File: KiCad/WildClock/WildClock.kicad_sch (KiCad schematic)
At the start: 33 parts, among them Q1 CA1, Q2 CA2, Q3 CA3, Q4 CA4, SW1 SWUP, SW2 SWDOWN, SW3 SWOK, U1 ESP32-C3-MINI-1, U3 74HC595, U4 TiltSensor

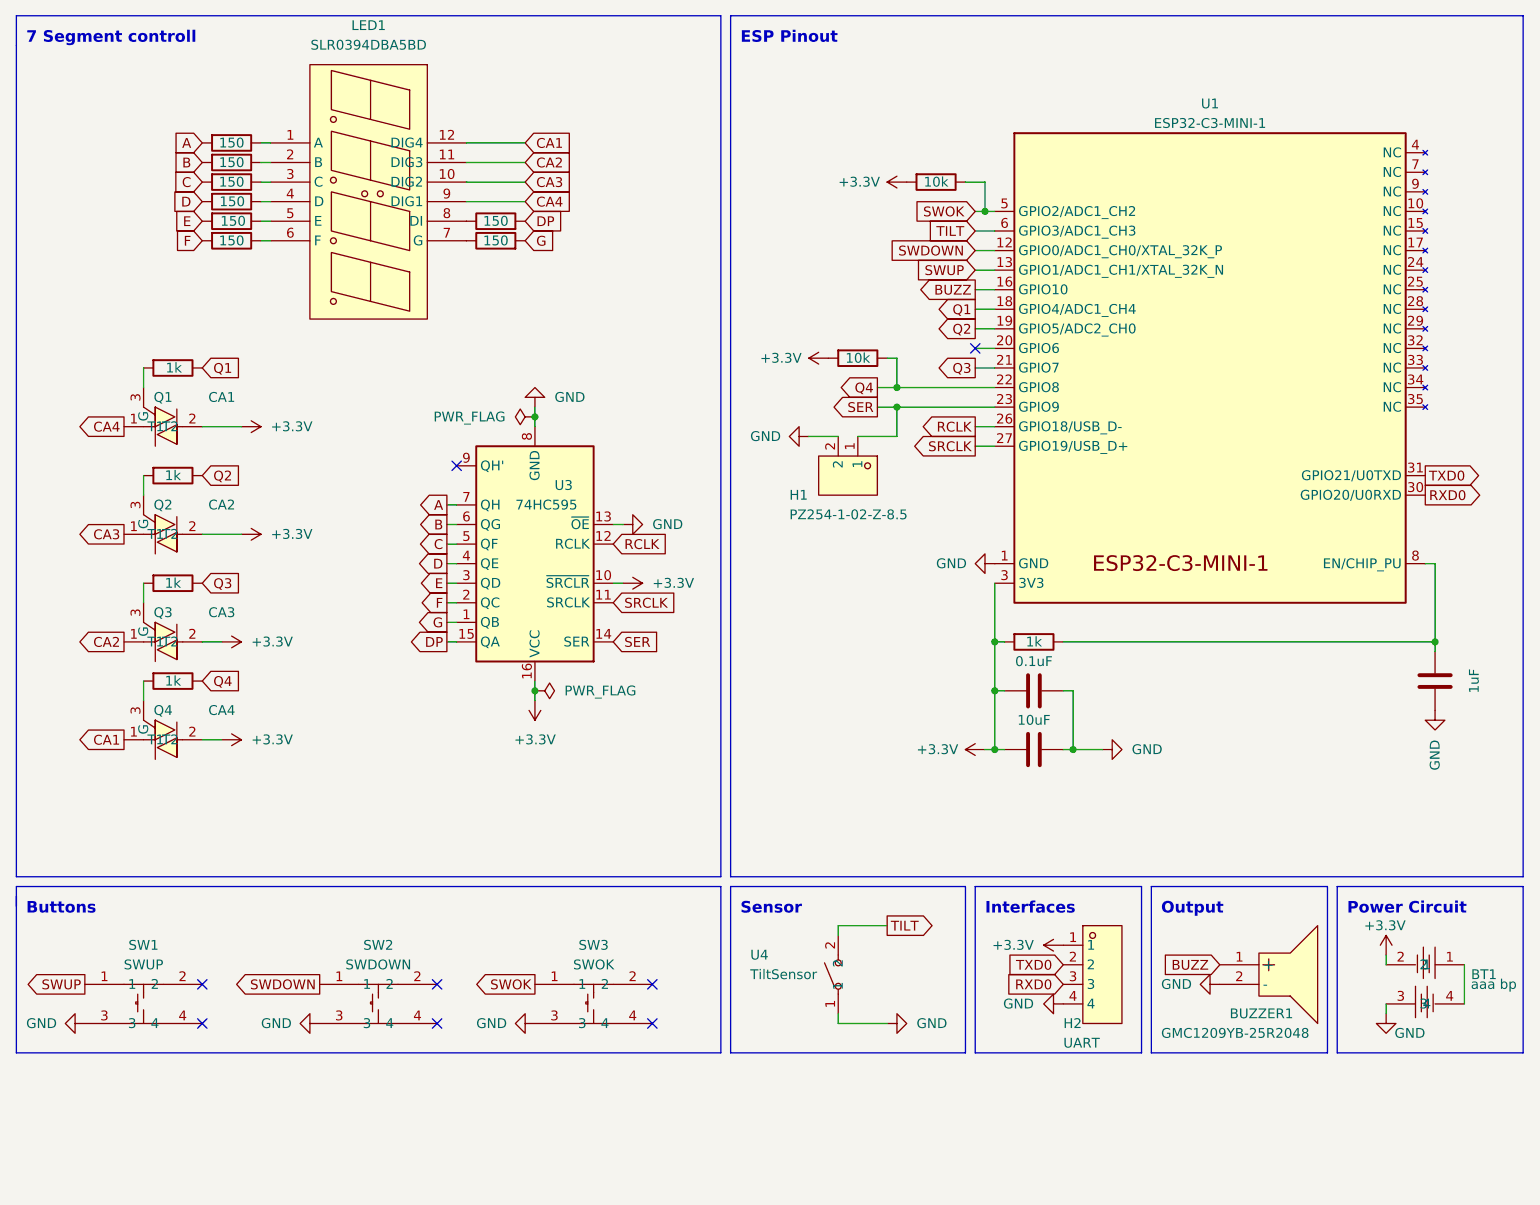
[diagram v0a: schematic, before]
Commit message: implemented maxis changes
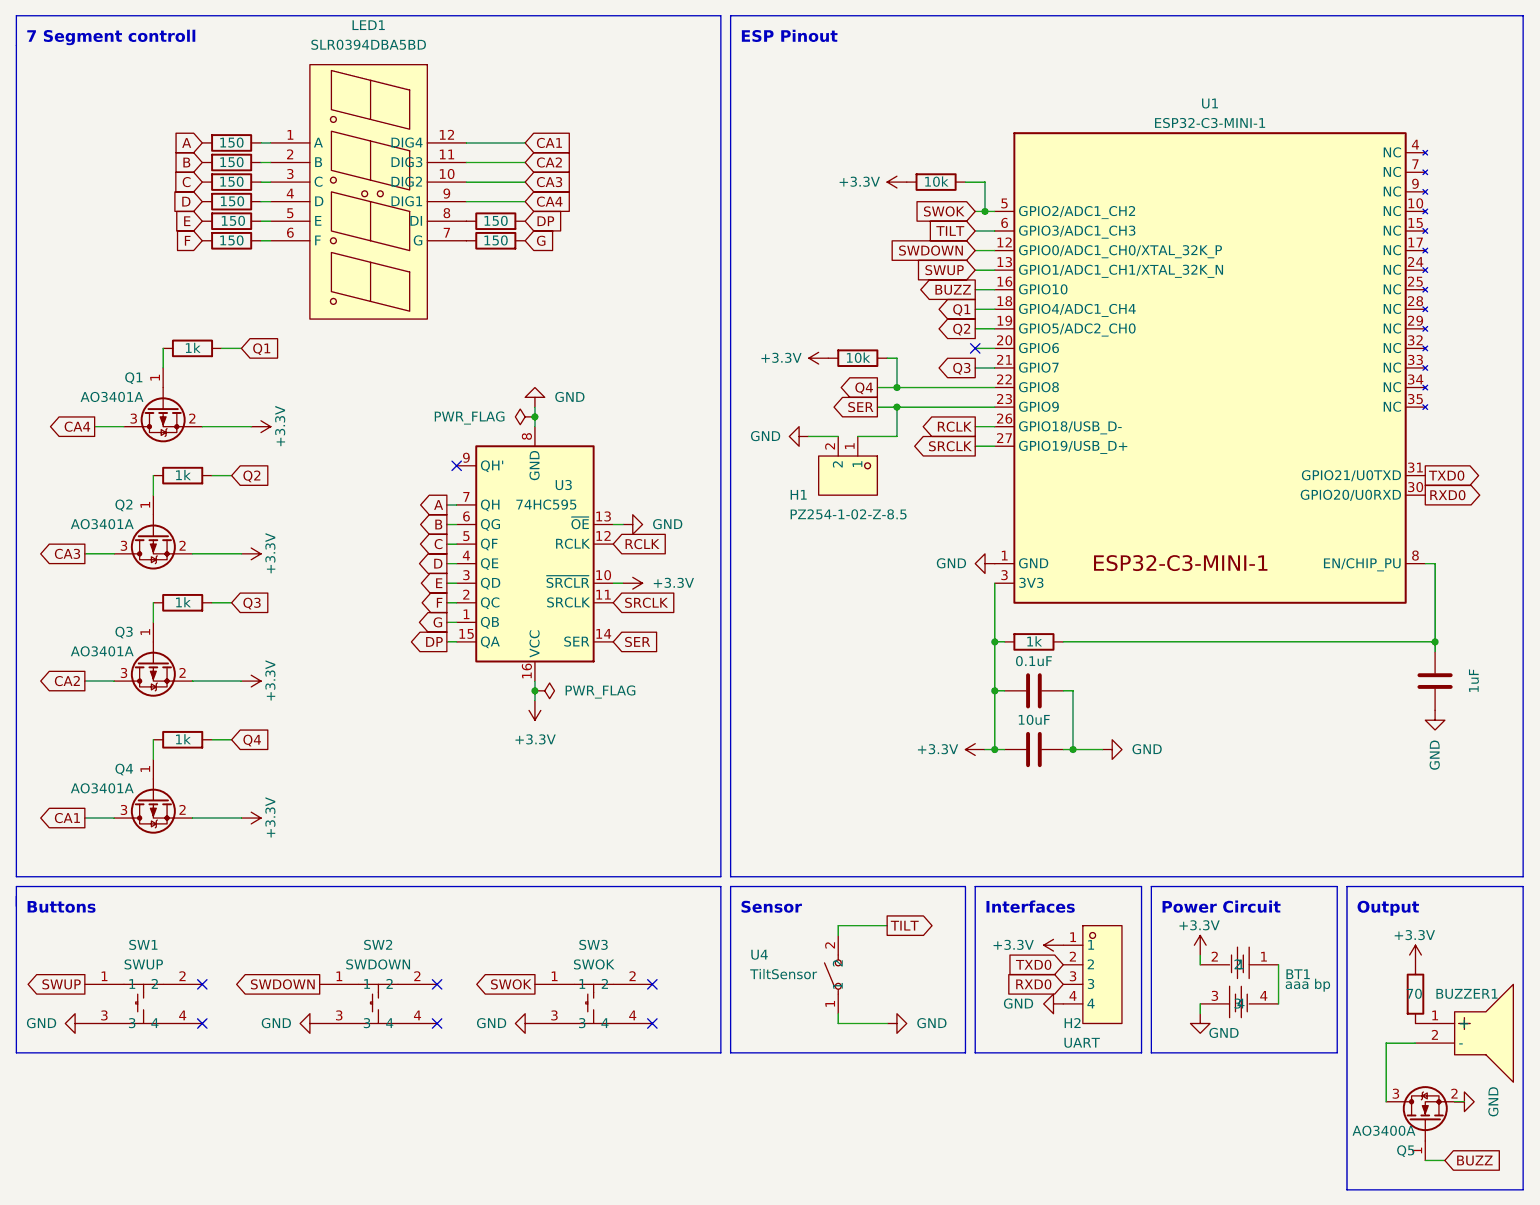
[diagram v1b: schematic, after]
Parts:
- removed Q1: CA1, easyeda2kicad:SOT-23-3_L2.9-W1.3-P1.90-LS2.4-BR-CW, symbol easyeda2kicad:BT169-23
- removed Q2: CA2, easyeda2kicad:SOT-23-3_L2.9-W1.3-P1.90-LS2.4-BR-CW, symbol easyeda2kicad:BT169-23
- removed Q3: CA3, easyeda2kicad:SOT-23-3_L2.9-W1.3-P1.90-LS2.4-BR-CW, symbol easyeda2kicad:BT169-23
- removed Q4: CA4, easyeda2kicad:SOT-23-3_L2.9-W1.3-P1.90-LS2.4-BR-CW, symbol easyeda2kicad:BT169-23
- added Q1, Q2, Q3, Q4: AO3401A, Package_TO_SOT_SMD:SOT-23, symbol Transistor_FET:AO3401A
- added Q5: AO3400A, Package_TO_SOT_SMD:SOT-23, symbol Transistor_FET:AO3400A
- added R5: 1k, Resistor_SMD:R_0805_2012Metric, symbol Device:R
- R2: value 1k -> 70
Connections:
- net +3.3V: now also R2.1, Q1.2 (S), Q2.2 (S), Q3.2 (S), Q4.2 (S)
- net BUZZ: now also Q5.1 (G); no longer BUZZER1.1 (+)
- net CA1: now also Q4.3 (D)
- net CA2: now also Q3.3 (D)
- net CA3: now also Q2.3 (D)
- net CA4: now also Q1.3 (D)
- net GND: now also Q5.2 (S); no longer BUZZER1.2 (-)
- net Q1: now also R1.2; no longer R1.1
- net Q2: now also R3.2; no longer R2.1
- net Q3: now also R4.2; no longer R3.1
- net Q4: now also R5.2; no longer R4.1
- net at R2.2: now also BUZZER1.1 (+)
- new net: Q2.1 (G), R3.1
- new net: Q1.1 (G), R1.1
- new net: Q4.1 (G), R5.1
- new net: Q3.1 (G), R4.1
- new net: BUZZER1.2 (-), Q5.3 (D)
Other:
- moved on the sheet: BT1, BUZZER1
